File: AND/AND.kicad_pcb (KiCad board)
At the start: 2 copper layers, 33.7 x 17.8 mm, 10 parts

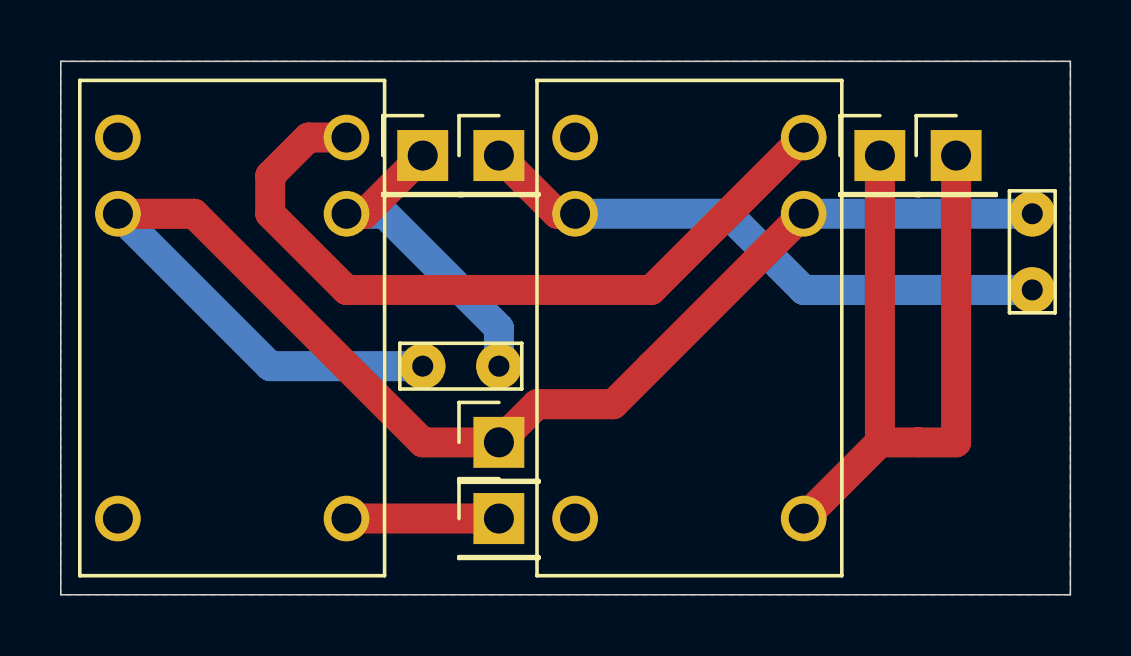
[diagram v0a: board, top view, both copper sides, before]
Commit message: Add files via upload
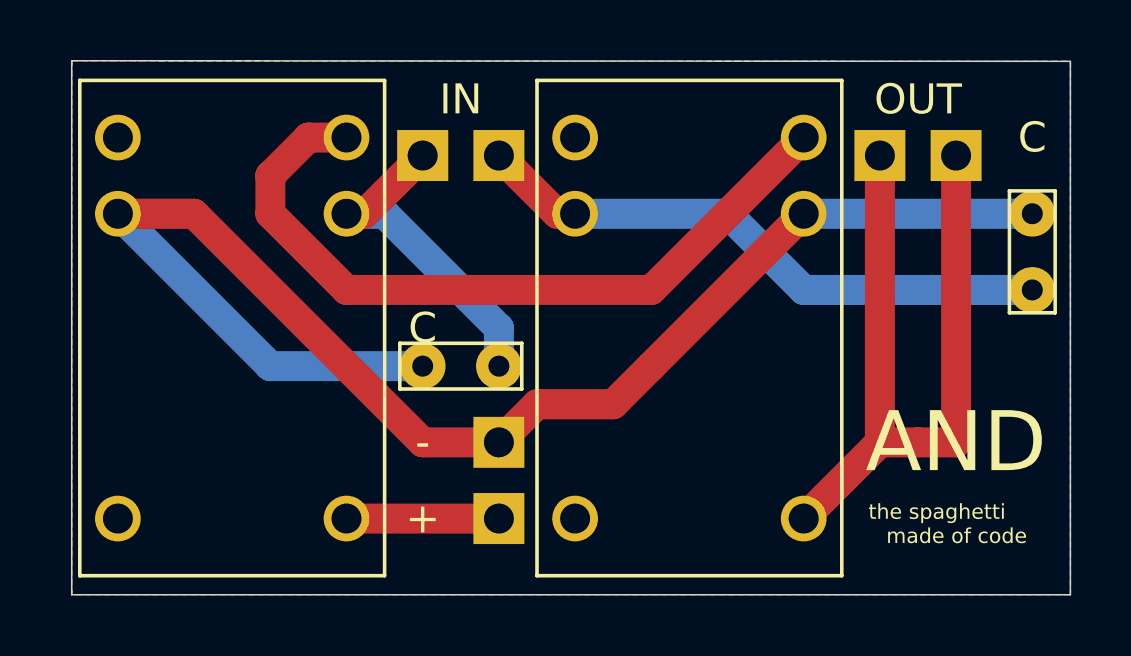
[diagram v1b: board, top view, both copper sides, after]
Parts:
- REF** (x6): moved to B.Cu
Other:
- board size 33.7 x 17.8 mm -> 33.3 x 17.8 mm
- board text added: "the spaghetti made of code"
- board text removed: "the spaghetti made of codes"
